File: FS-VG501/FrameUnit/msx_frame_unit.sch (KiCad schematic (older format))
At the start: 244 parts, among them CN1 Conn_01x02, CN2 Conn_01x10, CN3 Conn_01x04, CN4 Conn_01x10, CN5 Conn_01x10, CN7 Conn_01x06, CN8 Conn_01x06, CN9 Conn_01x02, IC1 74LS245, IC10 74S08, IC11 74LS273, IC12 74LS273, IC13 74LS138, IC14 74LS04, IC15 74LS11, IC16 74S124/74LS629, IC17 74LS153, IC18 74LS153, IC19 74LS153, IC2 74LS244, IC20 74LS08, IC21 SLA6430, IC22 74LS32, IC23 SLA6170, IC24 TC15G008AP, IC24 TC5081AP, IC25 74HC174, IC25 TC15G008AP, IC26 74LS153, IC27 74LS153, IC27 TC15G008AP, IC28 74LS123, IC28 TC15G008AP, IC29 74LS32, IC3 74LS123, IC30 TC15G008AP, IC31 74HC174, IC32 74LS153, IC33 74LS153, IC36 74LS04, IC39 74LS54, IC4 74LS09, IC40 74LS54, IC41 74HC174, IC42 74LS153, IC43 74LS153, IC44 74LS04, IC45 74LS54, IC46 74LS54, IC47 DRAM_4464, IC48 DRAM_4464, IC49 DRAM_4464, IC5 MB40576, IC50 DRAM_4464, IC51 DRAM_4464, IC52 DRAM_4464, IC53 DRAM_4464, IC54 DRAM_4464, IC55 DRAM_4464, IC56 DRAM_4464, IC57 DRAM_4464, IC58 DRAM_4464, IC59 DRAM_4464, IC6 MB40576, IC60 DRAM_4464, IC61 DRAM_4464, IC62 DRAM_4464, IC63 DRAM_4464, IC64 DRAM_4464, IC65 DRAM_4464, IC66 DRAM_4464, IC67 DRAM_4164, IC68 DRAM_4164, IC69 DRAM_4164, IC7 MB40576, IC70 DRAM_4164, IC8 74LS32, IC9 74LS10, Q1 A564_PNP, Q10 C1684_NPN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

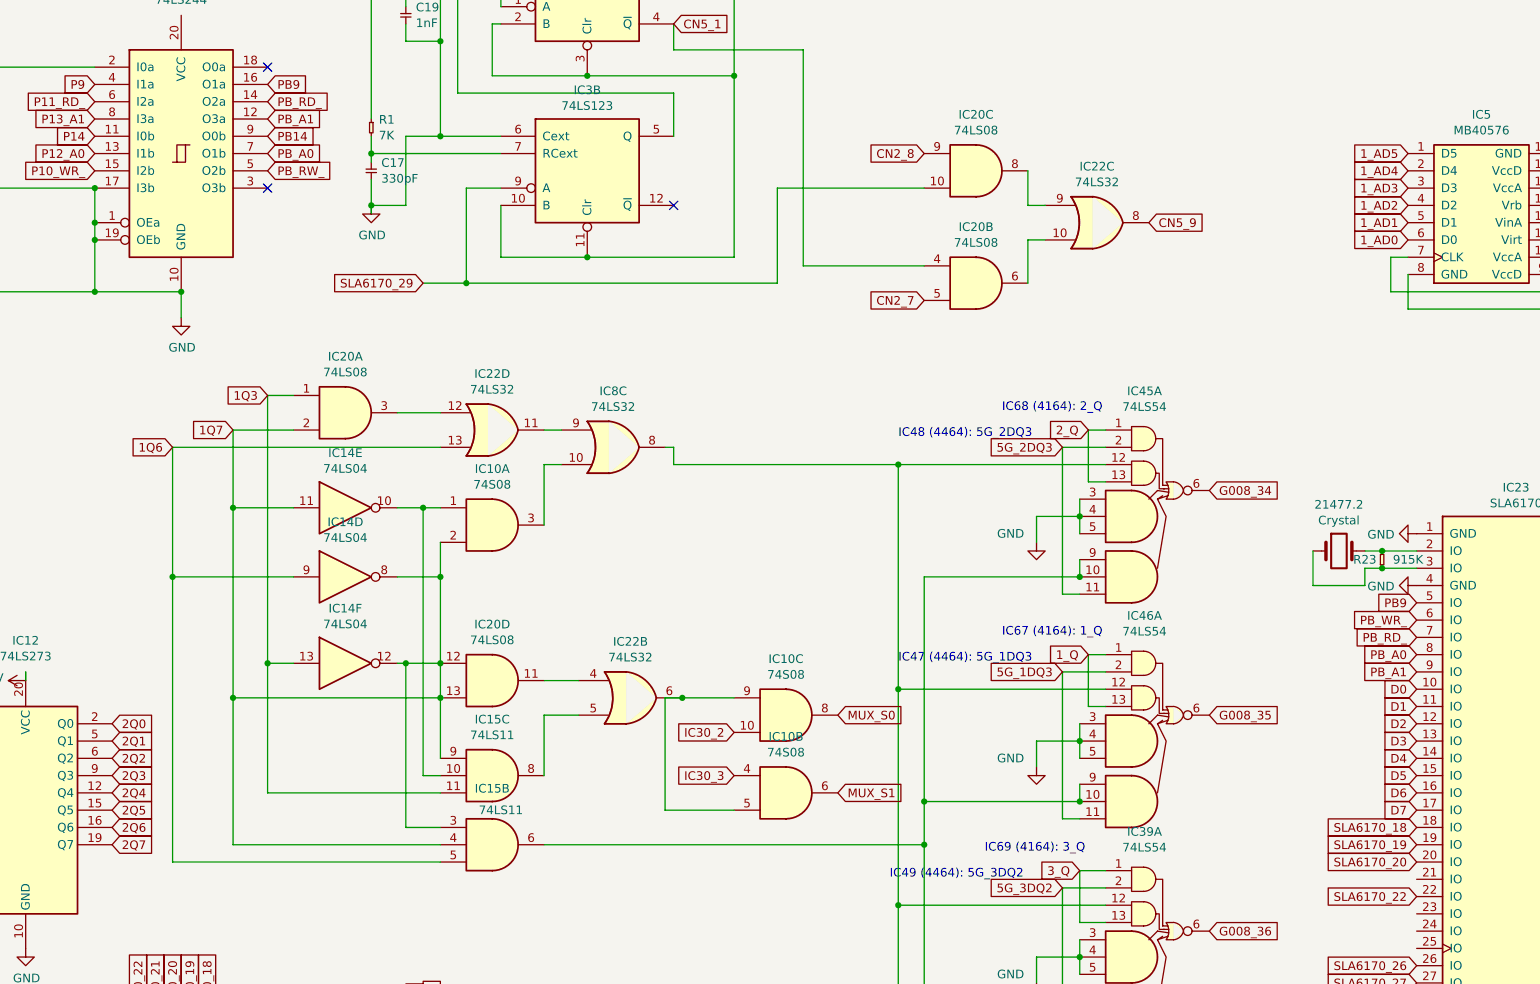
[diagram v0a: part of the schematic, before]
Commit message: Add files via upload
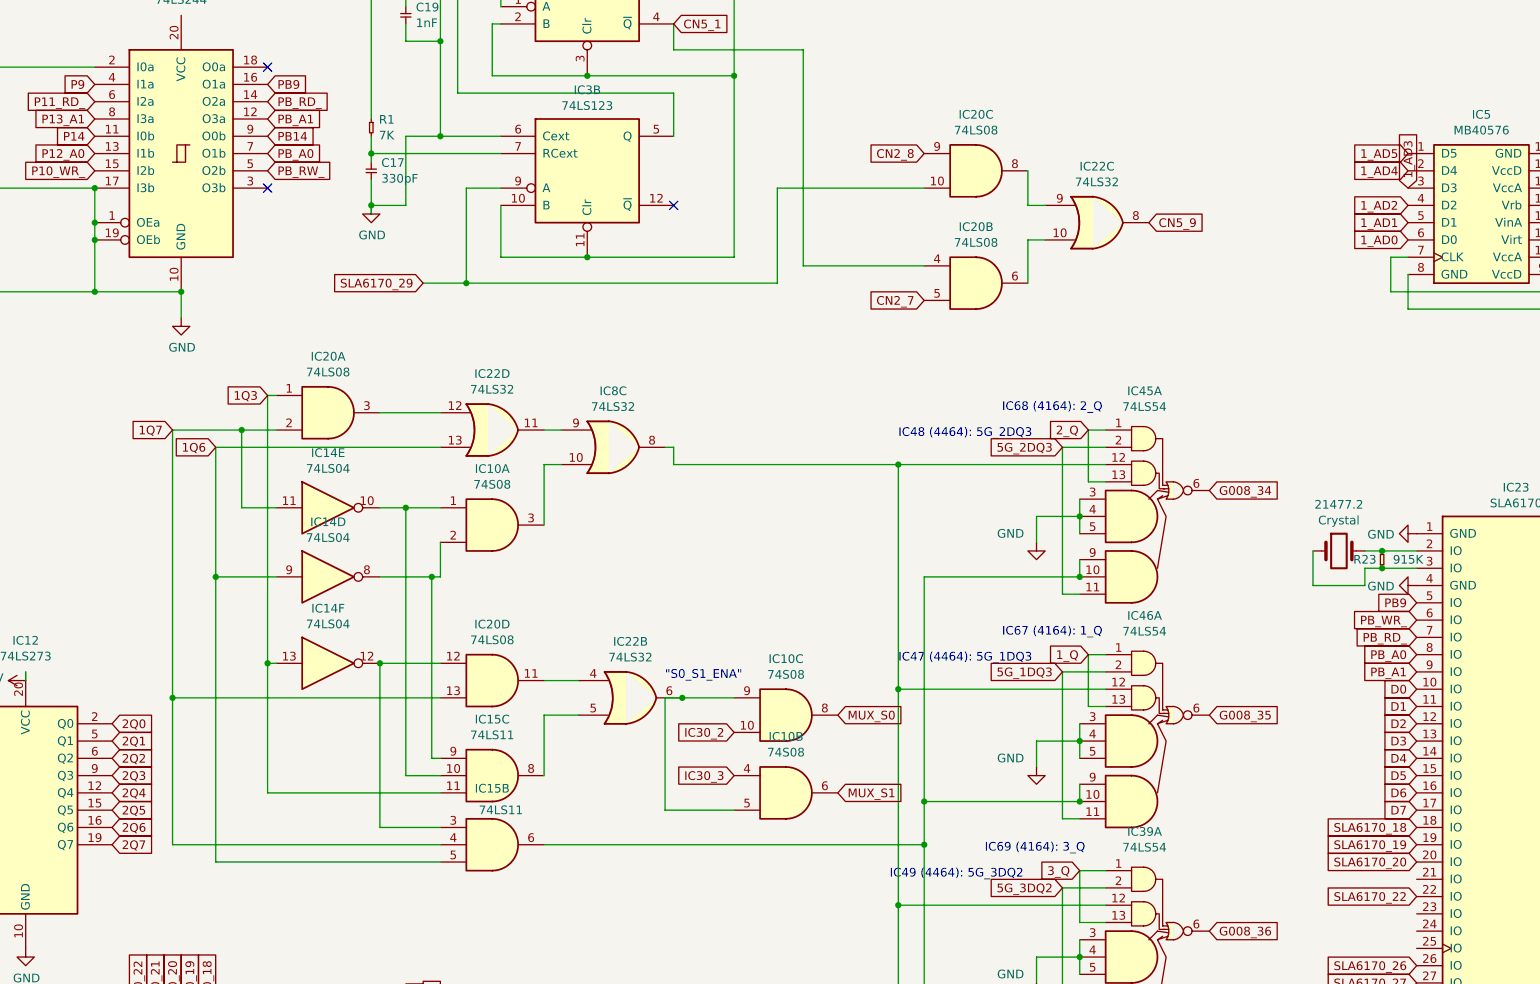
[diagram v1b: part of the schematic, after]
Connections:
- net 1Q7: no longer IC10.2, IC14.12, IC14.8, IC15.3, IC15.9, IC20.12
- new net: IC10.2, IC14.8, IC15.9
- new net: IC14.12, IC15.3, IC20.12
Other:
- note added: ""S0_S1_ENA""
- moved on the sheet: IC14D, IC14E, IC14F, IC20A
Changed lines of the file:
@@
 L 74xx:74LS04 IC14
 U 4 1 606EB0DC
-P 16200 8350
-F 0 "IC14" H 16200 8667 50  0000 C CNN
-F 1 "74LS04" H 16200 8576 50  0000 C CNN
-F 2 "" H 16200 8350 50  0001 C CNN
-F 3 "http://www.ti.com/lit/gpn/sn74LS04" H 16200 8350 50  0001 C CNN
-	4    16200 8350
+P 16100 8350
+F 0 "IC14" H 16100 8667 50  0000 C CNN
+F 1 "74LS04" H 16100 8576 50  0000 C CNN
+F 2 "" H 16100 8350 50  0001 C CNN
+F 3 "http://www.ti.com/lit/gpn/sn74LS04" H 16100 8350 50  0001 C CNN
+	4    16100 8350
 	1    0    0    -1
 $EndComp
@@
 L 74xx:74LS04 IC14
 U 5 1 606ECB6B
-P 16200 7950
-F 0 "IC14" H 16200 8267 50  0000 C CNN
-F 1 "74LS04" H 16200 8176 50  0000 C CNN
-F 2 "" H 16200 7950 50  0001 C CNN
-F 3 "http://www.ti.com/lit/gpn/sn74LS04" H 16200 7950 50  0001 C CNN
-	5    16200 7950
+P 16100 7950
+F 0 "IC14" H 16100 8267 50  0000 C CNN
+F 1 "74LS04" H 16100 8176 50  0000 C CNN
+F 2 "" H 16100 7950 50  0001 C CNN
+F 3 "http://www.ti.com/lit/gpn/sn74LS04" H 16100 7950 50  0001 C CNN
+	5    16100 7950
 	1    0    0    -1
 $EndComp
@@
 L 74xx:74LS04 IC14
 U 6 1 606EE556
-P 16200 8850
-F 0 "IC14" H 16200 9167 50  0000 C CNN
-F 1 "74LS04" H 16200 9076 50  0000 C CNN
-F 2 "" H 16200 8850 50  0001 C CNN
-F 3 "http://www.ti.com/lit/gpn/sn74LS04" H 16200 8850 50  0001 C CNN
-	6    16200 8850
+P 16100 8850
+F 0 "IC14" H 16100 9167 50  0000 C CNN
+F 1 "74LS04" H 16100 9076 50  0000 C CNN
+F 2 "" H 16100 8850 50  0001 C CNN
+F 3 "http://www.ti.com/lit/gpn/sn74LS04" H 16100 8850 50  0001 C CNN
+	6    16100 8850
 	1    0    0    -1
 $EndComp
@@
 L 74xx:74LS08 IC20
 U 1 1 6071264F
-P 16200 7400
-F 0 "IC20" H 16200 7725 50  0000 C CNN
-F 1 "74LS08" H 16200 7634 50  0000 C CNN
-F 2 "" H 16200 7400 50  0001 C CNN
-F 3 "http://www.ti.com/lit/gpn/sn74LS08" H 16200 7400 50  0001 C CNN
-	1    16200 7400
+P 16100 7400
+F 0 "IC20" H 16100 7725 50  0000 C CNN
+F 1 "74LS08" H 16100 7634 50  0000 C CNN
+F 2 "" H 16100 7400 50  0001 C CNN
+F 3 "http://www.ti.com/lit/gpn/sn74LS08" H 16100 7400 50  0001 C CNN
+	1    16100 7400
 	1    0    0    -1
 $EndComp
@@
 Wire Wire Line
 	17350 7500 17450 7500
-Text GLabel 15550 7500 0    50   Input ~ 0
+Text GLabel 15200 7500 0    50   Input ~ 0
 1Q7
 Wire Wire Line
@@
 Text GLabel 22350 6000 0    50   Input ~ 0
 1_AD4
-Text GLabel 22350 6100 0    50   Input ~ 0
+Text GLabel 22350 6100 1    50   Input ~ 0
 1_AD3
 Text GLabel 22350 6200 0    50   Input ~ 0
@@
 Text GLabel 9350 5600 2    50   Input ~ 0
 CN3_3
-Text GLabel 15200 7600 0    50   Input ~ 0
+Text GLabel 15450 7600 0    50   Input ~ 0
 1Q6
 Wire Wire Line
@@
 Wire Wire Line
 	17350 9150 17550 9150
-Wire Wire Line
-	16750 9500 16650 9500
 $Comp
 L 74xx:74LS54 IC45
@@
 $EndComp
 Wire Wire Line
-	16750 9800 16550 9800
-Wire Wire Line
-	16650 7950 16650 9500
+	16550 7950 16550 9500
 Wire Wire Line
 	16750 8350 16750 8150
 Wire Wire Line
-	16750 9050 15550 9050
-Wire Wire Line
-	15550 7950 15900 7950
-Wire Wire Line
-	15550 9900 16750 9900
-Connection ~ 15550 9050
-Wire Wire Line
-	15550 9050 15550 9900
-Wire Wire Line
-	15550 7950 15550 9050
-Wire Wire Line
-	16750 10000 15200 10000
-Wire Wire Line
-	15200 7600 16750 7600
-Wire Wire Line
-	15200 7600 15200 8350
-Wire Wire Line
-	15900 8350 15200 8350
-Connection ~ 15200 8350
-Wire Wire Line
-	15200 8350 15200 10000
-Wire Wire Line
-	16500 7400 16750 7400
+	16750 10000 15450 10000
 Wire Wire Line
-	15900 7300 15750 7300
+	15450 7600 15450 8350
 Wire Wire Line
-	15750 7300 15750 8850
+	15450 8350 15450 10000
 Connection ~ 15750 8850
 Wire Wire Line
@@
 	15750 9600 16750 9600
 Wire Wire Line
-	15900 7500 15550 7500
-Wire Wire Line
-	15550 7950 15550 7500
-Connection ~ 15550 7950
-Wire Wire Line
-	16500 8850 16550 8850
-Wire Wire Line
-	16550 8850 16550 9800
-Connection ~ 16750 8350
-Wire Wire Line
-	16750 8350 16750 8850
-Wire Wire Line
-	16500 8350 16750 8350
-Connection ~ 16650 7950
+	16400 8850 16400 9800
 Wire Wire Line
-	16650 7950 16750 7950
-Wire Wire Line
-	16500 7950 16650 7950
-Connection ~ 16550 8850
-Wire Wire Line
-	16550 8850 16750 8850
-Wire Wire Line
-	15750 8850 15900 8850
+	15750 8850 15800 8850
 Text GLabel 6750 10500 0    50   Input ~ 0
 MUX_S0
@@
 Wire Wire Line
 	20450 10800 20450 10900
-Connection ~ 16750 8850
-Wire Wire Line
-	16750 8850 16750 9050
-Connection ~ 16750 9050
-Wire Wire Line
-	16750 9050 16750 9400
 Wire Wire Line
 	18150 9050 18450 9050
@@
 Text Notes 9050 17300 0    50   ~ 0
 "1DAQ5"
+Wire Wire Line
+	16700 9400 16750 9400
+Wire Wire Line
+	16700 8350 16700 9400
+Connection ~ 16700 8350
+Wire Wire Line
+	16700 8350 16750 8350
+Wire Wire Line
+	15800 8350 15450 8350
+Wire Wire Line
+	15800 7300 15750 7300
+Wire Wire Line
+	16400 7400 16750 7400
+Wire Wire Line
+	16400 7950 16550 7950
+Wire Wire Line
+	16400 8350 16700 8350
+Connection ~ 16400 8850
+Wire Wire Line
+	16400 8850 16750 8850
+Connection ~ 16550 7950
+Wire Wire Line
+	16550 7950 16750 7950
+Wire Wire Line
+	16550 9500 16750 9500
+Wire Wire Line
+	16400 9800 16750 9800
+Wire Wire Line
+	15450 7600 16750 7600
+Connection ~ 15450 8350
+Connection ~ 15200 9050
+Wire Wire Line
+	15200 9050 16750 9050
+Wire Wire Line
+	15200 7500 15200 9050
+Wire Wire Line
+	15200 9900 16750 9900
+Wire Wire Line
+	15200 9050 15200 9900
+Wire Wire Line
+	15200 7500 15600 7500
+Wire Wire Line
+	15750 7300 15750 8850
+Wire Wire Line
+	15800 7950 15600 7950
+Wire Wire Line
+	15600 7950 15600 7500
+Connection ~ 15600 7500
+Wire Wire Line
+	15600 7500 15800 7500
+Text Notes 18050 8950 0    50   ~ 0
+"S0_S1_ENA"
 $EndSCHEMATC
